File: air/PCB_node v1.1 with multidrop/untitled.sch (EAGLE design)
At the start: 113 parts, among them J1 10118193-0001LF, J2 10118193-0001LF, K1 351, K2 351, K3 SRD-05VDC-SL-C, K4 351, Q1 MMBT3904, Q10 S9013, Q2 MMBT3904, Q3 12MHz, Q4 S9013, Q5 S9013, Q6 S9013, Q7 12MHz, Q8 MMBT3904, Q9 MMBT3904, U1 CH340G, U10 ADS1115IDGSR, U11 PC817X2NIP0F, U2 ESP32-WROOM-32D, U3 AMS1117, U4 PC817X2NIP0F, U5 PC817X2NIP0F, U6 PC817X2NIP0F, U7 CH340G, U8 AMS1117, U9 ESP32-WROOM-32D, X1 MSTBA2, X2 MSTBA2, X3 MSTBA4, X4 MSTBA3, X5 MSTBA2, X6 MSTBA4, X7 C-GRID-02-70543, X8 MSTBA2

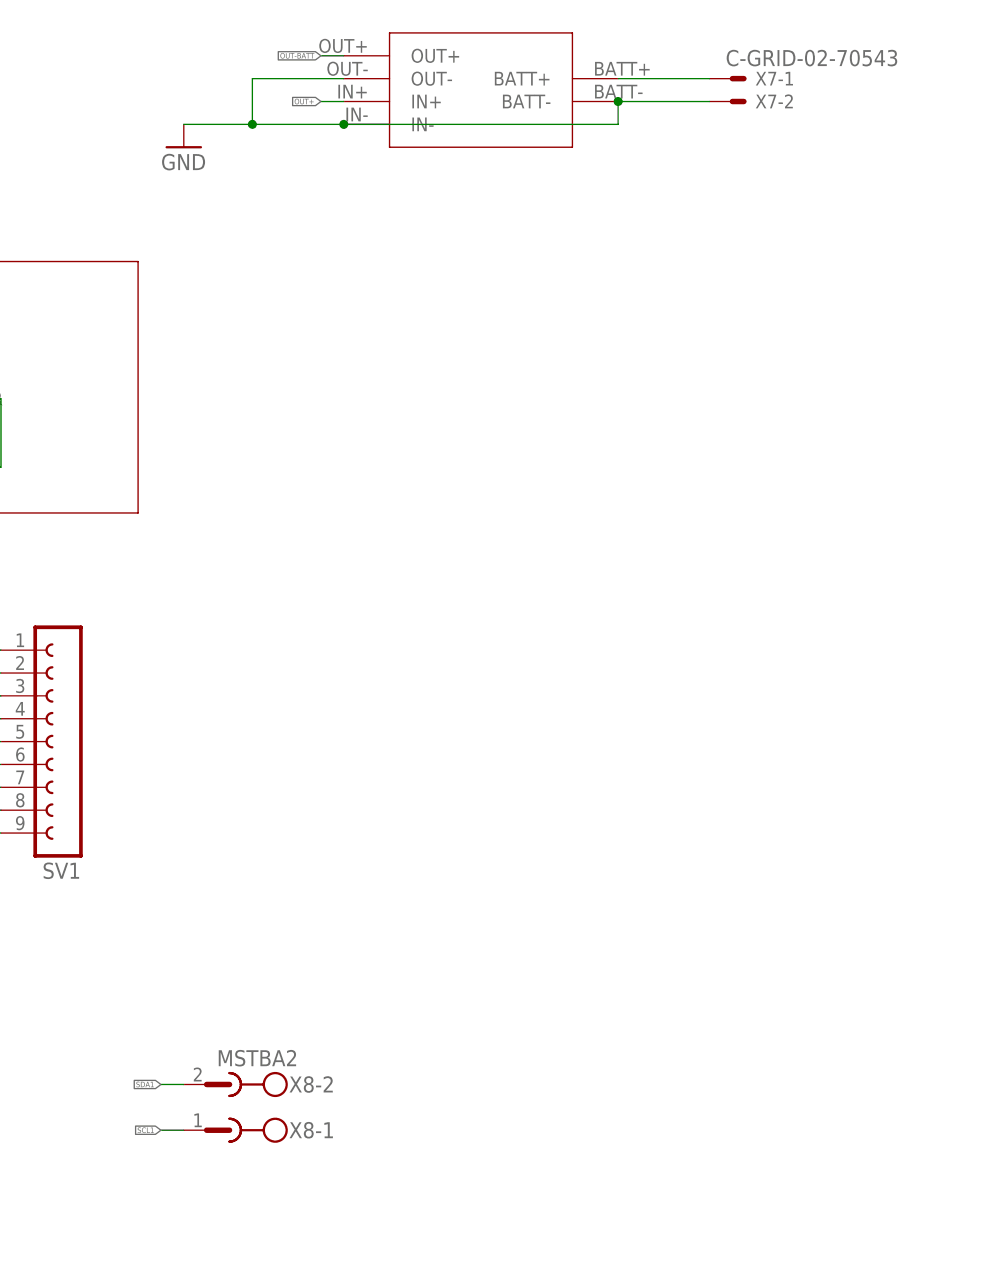
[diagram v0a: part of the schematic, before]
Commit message: menambah GPS chip
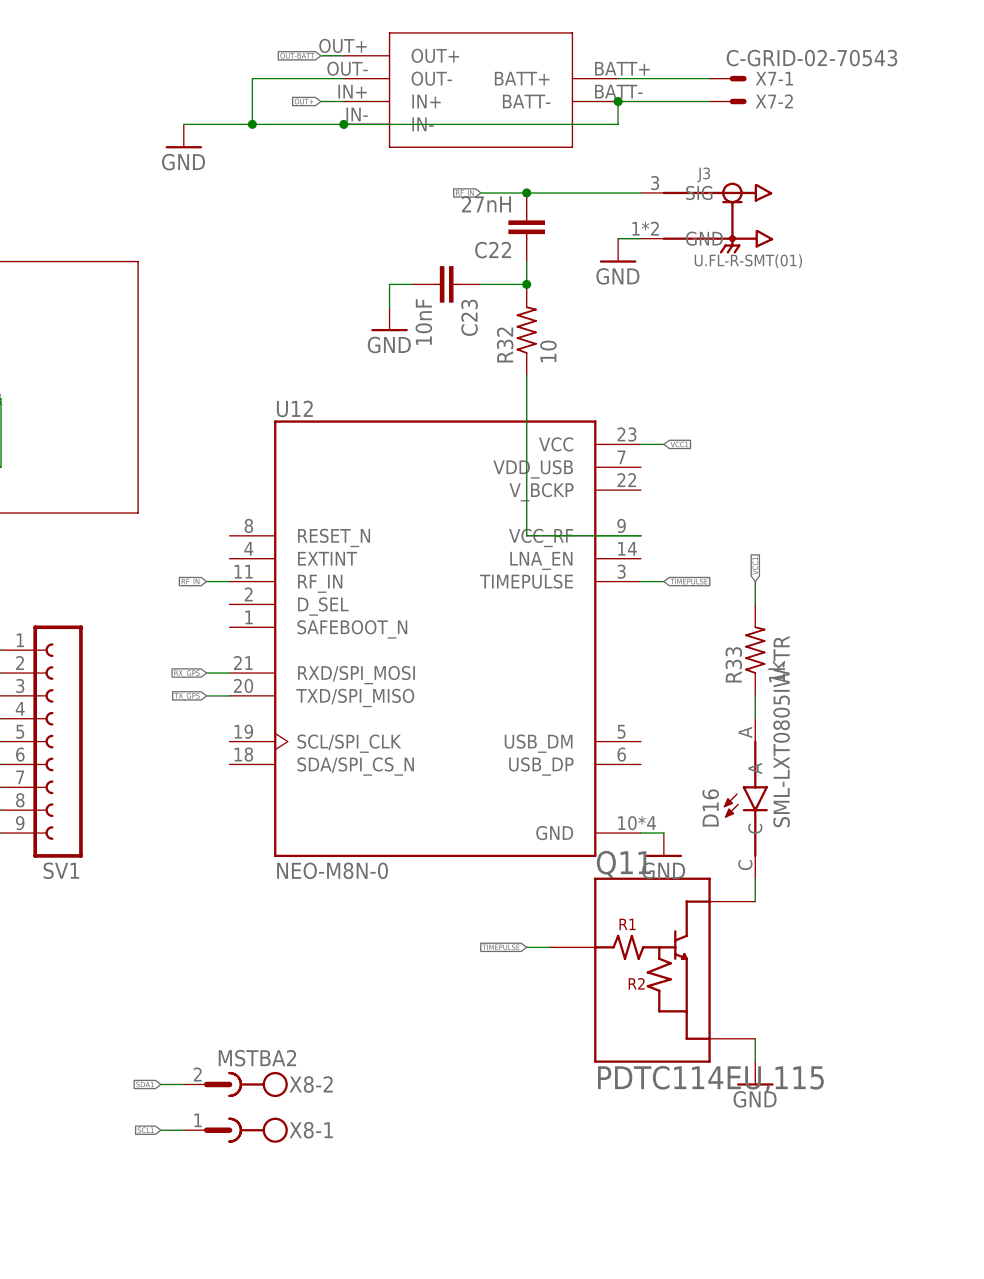
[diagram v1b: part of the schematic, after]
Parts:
- added C22: 27nH, rcl:C-EUC0805K
- added C23: 10nF, rcl:C-EUC0805K
- added D16: SML-LXT0805IW-TR, SML-LXT0805IW-TR:SML-LXT0805IW-TR
- added J3: U.FL-R-SMT(01), U.FL-R-SMT_01_:U.FL-R-SMT(01)
- added Q11: PDTC114EU,115, PDTC114EU_115:PDTC114EU,115
- added R32: 10, rcl:R-US_M0805
- added R33: 1k, rcl:R-US_M0805
- added U12: NEO-M8N-0, NEO-M8N-0:NEO-M8N-0
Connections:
- new net N$36: C22.1, C23.1, R32.2
- new net N$37: R32.1, U12.VCC_RF
- new net N$38: D16.C, Q11.OUTPUT
- new net N$39: D16.A, R33.1
- new net RF_IN: C22.2, J3.SIG, U12.RF_IN
- new net TIMEPULSE: Q11.INPUT, U12.TIMEPULSE
- net GND: now also C23.2, J3.GND, Q11.GND, U12.GND
- net RX_GPS: now also U12.RXD/SPI_MOSI
- net TX_GPS: now also U12.TXD/SPI_MISO
- net VCC1: now also R33.2, U12.VCC
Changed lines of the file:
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@@
 <part name="P+7" library="supply1" library_urn="urn:adsk.eagle:library:371" deviceset="VCC" device=""/>
 <part name="GND33" library="supply1" library_urn="urn:adsk.eagle:library:371" deviceset="GND" device=""/>
+<part name="U12" library="NEO-M8N-0" deviceset="NEO-M8N-0" device=""/>
+<part name="GND34" library="supply1" library_urn="urn:adsk.eagle:library:371" deviceset="GND" device=""/>
+<part name="J3" library="U.FL-R-SMT_01_" deviceset="U.FL-R-SMT(01)" device=""/>
+<part name="GND35" library="supply1" library_urn="urn:adsk.eagle:library:371" deviceset="GND" device=""/>
+<part name="C22" library="rcl" library_urn="urn:adsk.eagle:library:334" deviceset="C-EU" device="C0805K" package3d_urn="urn:adsk.eagle:package:23681/2" value="27nH"/>
+<part name="R32" library="rcl" library_urn="urn:adsk.eagle:library:334" deviceset="R-US_" device="M0805" package3d_urn="urn:adsk.eagle:package:23556/2" value="10"/>
+<part name="Q11" library="PDTC114EU_115" deviceset="PDTC114EU,115" device=""/>
+<part name="C23" library="rcl" library_urn="urn:adsk.eagle:library:334" deviceset="C-EU" device="C0805K" package3d_urn="urn:adsk.eagle:package:23681/2" value="10nF"/>
+<part name="GND36" library="supply1" library_urn="urn:adsk.eagle:library:371" deviceset="GND" device=""/>
+<part name="GND37" library="supply1" library_urn="urn:adsk.eagle:library:371" deviceset="GND" device=""/>
+<part name="D16" library="SML-LXT0805IW-TR" deviceset="SML-LXT0805IW-TR" device=""/>
+<part name="R33" library="rcl" library_urn="urn:adsk.eagle:library:334" deviceset="R-US_" device="M0805" package3d_urn="urn:adsk.eagle:package:23556/2" value="1k"/>
 </parts>
 <sheets>
@@
 <instance part="GND33" gate="1" x="78.74" y="172.72" smashed="yes">
 <attribute name="VALUE" x="76.2" y="170.18" size="1.778" layer="96"/>
+</instance>
+<instance part="U12" gate="G$1" x="287.02" y="99.06" smashed="yes">
+<attribute name="NAME" x="269.2361" y="122.4338" size="1.77845" layer="95"/>
+<attribute name="VALUE" x="269.2355" y="71.1126" size="1.77851875" layer="96"/>
+</instance>
+<instance part="GND34" gate="1" x="312.42" y="73.66" smashed="yes">
+<attribute name="VALUE" x="309.88" y="71.12" size="1.778" layer="96"/>
+</instance>
+<instance part="J3" gate="G$1" x="320.04" y="144.78" smashed="yes">
+<attribute name="NAME" x="316.22143125" y="148.85313125" size="1.27285" layer="95"/>
+<attribute name="VALUE" x="315.71218125" y="139.1793" size="1.27288125" layer="96"/>
+</instance>
+<instance part="GND35" gate="1" x="307.34" y="139.7" smashed="yes">
+<attribute name="VALUE" x="304.8" y="137.16" size="1.778" layer="96"/>
+</instance>
+<instance part="C22" gate="G$1" x="297.18" y="142.24" smashed="yes" rot="R180">
+<attribute name="NAME" x="295.656" y="141.859" size="1.778" layer="95" rot="R180"/>
+<attribute name="VALUE" x="295.656" y="146.939" size="1.778" layer="96" rot="R180"/>
+</instance>
+<instance part="R32" gate="G$1" x="297.18" y="132.08" smashed="yes" rot="R90">
+<attribute name="NAME" x="295.6814" y="128.27" size="1.778" layer="95" rot="R90"/>
+<attribute name="VALUE" x="300.482" y="128.27" size="1.778" layer="96" rot="R90"/>
+</instance>
+<instance part="Q11" gate="G$1" x="312.42" y="60.96" smashed="yes">
+<attribute name="NAME" x="304.7945" y="71.6357" size="2.54183125" layer="95"/>
+<attribute name="VALUE" x="304.79283125" y="47.7396" size="2.542390625" layer="96"/>
+</instance>
+<instance part="C23" gate="G$1" x="289.56" y="137.16" smashed="yes" rot="R270">
+<attribute name="NAME" x="289.941" y="135.636" size="1.778" layer="95" rot="R270"/>
+<attribute name="VALUE" x="284.861" y="135.636" size="1.778" layer="96" rot="R270"/>
+</instance>
+<instance part="GND36" gate="1" x="281.94" y="132.08" smashed="yes">
+<attribute name="VALUE" x="279.4" y="129.54" size="1.778" layer="96"/>
+</instance>
+<instance part="GND37" gate="1" x="322.58" y="48.26" smashed="yes">
+<attribute name="VALUE" x="320.04" y="45.72" size="1.778" layer="96"/>
+</instance>
+<instance part="D16" gate="G$1" x="322.58" y="78.74" smashed="yes" rot="R90">
+<attribute name="NAME" x="318.50973125" y="76.70486875" size="1.780740625" layer="95" rot="R90"/>
+<attribute name="VALUE" x="326.39315" y="76.70631875" size="1.77946875" layer="96" rot="R90"/>
+</instance>
+<instance part="R33" gate="G$1" x="322.58" y="96.52" smashed="yes" rot="R90">
+<attribute name="NAME" x="321.0814" y="92.71" size="1.778" layer="95" rot="R90"/>
+<attribute name="VALUE" x="325.882" y="92.71" size="1.778" layer="96" rot="R90"/>
 </instance>
 </instances>
@@
 <wire x1="91.44" y1="175.26" x2="78.74" y2="175.26" width="0.1524" layer="91"/>
 </segment>
+<segment>
+<pinref part="U12" gate="G$1" pin="GND"/>
+<wire x1="309.88" y1="76.2" x2="312.42" y2="76.2" width="0.1524" layer="91"/>
+<pinref part="GND34" gate="1" pin="GND"/>
+</segment>
+<segment>
+<pinref part="J3" gate="G$1" pin="GND"/>
+<wire x1="309.88" y1="142.24" x2="307.34" y2="142.24" width="0.1524" layer="91"/>
+<pinref part="GND35" gate="1" pin="GND"/>
+</segment>
+<segment>
+<pinref part="C23" gate="G$1" pin="2"/>
+<pinref part="GND36" gate="1" pin="GND"/>
+<wire x1="284.48" y1="137.16" x2="281.94" y2="137.16" width="0.1524" layer="91"/>
+<wire x1="281.94" y1="137.16" x2="281.94" y2="134.62" width="0.1524" layer="91"/>
+</segment>
+<segment>
+<pinref part="Q11" gate="G$1" pin="GND"/>
+<pinref part="GND37" gate="1" pin="GND"/>
+<wire x1="322.58" y1="53.34" x2="322.58" y2="50.8" width="0.1524" layer="91"/>
+</segment>
 </net>
 <net name="VUSB" class="0">
@@
 <label x="215.9" y="91.44" size="0.6096" layer="95" rot="R270" xref="yes"/>
 </segment>
+<segment>
+<pinref part="U12" gate="G$1" pin="VCC"/>
+<wire x1="309.88" y1="119.38" x2="312.42" y2="119.38" width="0.1524" layer="91"/>
+<label x="312.42" y="119.38" size="0.6096" layer="95" xref="yes"/>
+</segment>
+<segment>
+<pinref part="R33" gate="G$1" pin="2"/>
+<wire x1="322.58" y1="101.6" x2="322.58" y2="104.14" width="0.1524" layer="91"/>
+<label x="322.58" y="104.14" size="0.6096" layer="95" rot="R90" xref="yes"/>
+</segment>
 </net>
 <net name="RX_MICRO" class="0">
@@
 <label x="228.6" y="30.48" size="0.6096" layer="95" xref="yes"/>
 </segment>
+<segment>
+<pinref part="U12" gate="G$1" pin="RXD/SPI_MOSI"/>
+<wire x1="264.16" y1="93.98" x2="261.62" y2="93.98" width="0.1524" layer="91"/>
+<label x="261.62" y="93.98" size="0.6096" layer="95" rot="R180" xref="yes"/>
+</segment>
 </net>
 <net name="TX_GPS" class="0">
@@
 <wire x1="223.52" y1="45.72" x2="228.6" y2="45.72" width="0.1524" layer="91"/>
 <label x="228.6" y="45.72" size="0.6096" layer="95" xref="yes"/>
+</segment>
+<segment>
+<pinref part="U12" gate="G$1" pin="TXD/SPI_MISO"/>
+<wire x1="264.16" y1="91.44" x2="261.62" y2="91.44" width="0.1524" layer="91"/>
+<label x="261.62" y="91.44" size="0.6096" layer="95" rot="R180" xref="yes"/>
 </segment>
 </net>
@@
 </segment>
 </net>
+<net name="RF_IN" class="0">
+<segment>
+<pinref part="J3" gate="G$1" pin="SIG"/>
+<wire x1="309.88" y1="147.32" x2="297.18" y2="147.32" width="0.1524" layer="91"/>
+<pinref part="C22" gate="G$1" pin="2"/>
+<wire x1="297.18" y1="147.32" x2="292.1" y2="147.32" width="0.1524" layer="91"/>
+<junction x="297.18" y="147.32"/>
+<label x="292.1" y="147.32" size="0.6096" layer="95" rot="R180" xref="yes"/>
+</segment>
+<segment>
+<pinref part="U12" gate="G$1" pin="RF_IN"/>
+<wire x1="264.16" y1="104.14" x2="261.62" y2="104.14" width="0.1524" layer="91"/>
+<label x="261.62" y="104.14" size="0.6096" layer="95" rot="R180" xref="yes"/>
+</segment>
+</net>
+<net name="N$36" class="0">
+<segment>
+<pinref part="C22" gate="G$1" pin="1"/>
+<pinref part="R32" gate="G$1" pin="2"/>
+<wire x1="297.18" y1="139.7" x2="297.18" y2="137.16" width="0.1524" layer="91"/>
+<pinref part="C23" gate="G$1" pin="1"/>
+<wire x1="297.18" y1="137.16" x2="292.1" y2="137.16" width="0.1524" layer="91"/>
+<junction x="297.18" y="137.16"/>
+</segment>
+</net>
+<net name="N$37" class="0">
+<segment>
+<pinref part="R32" gate="G$1" pin="1"/>
+<pinref part="U12" gate="G$1" pin="VCC_RF"/>
+<wire x1="297.18" y1="127" x2="297.18" y2="109.22" width="0.1524" layer="91"/>
+<wire x1="297.18" y1="109.22" x2="309.88" y2="109.22" width="0.1524" layer="91"/>
+</segment>
+</net>
+<net name="TIMEPULSE" class="0">
+<segment>
+<pinref part="U12" gate="G$1" pin="TIMEPULSE"/>
+<wire x1="309.88" y1="104.14" x2="312.42" y2="104.14" width="0.1524" layer="91"/>
+<label x="312.42" y="104.14" size="0.6096" layer="95" xref="yes"/>
+</segment>
+<segment>
+<pinref part="Q11" gate="G$1" pin="INPUT"/>
+<wire x1="299.72" y1="63.5" x2="297.18" y2="63.5" width="0.1524" layer="91"/>
+<label x="297.18" y="63.5" size="0.6096" layer="95" rot="R180" xref="yes"/>
+</segment>
+</net>
+<net name="N$38" class="0">
+<segment>
+<pinref part="Q11" gate="G$1" pin="OUTPUT"/>
+<pinref part="D16" gate="G$1" pin="C"/>
+<wire x1="322.58" y1="68.58" x2="322.58" y2="71.12" width="0.1524" layer="91"/>
+</segment>
+</net>
+<net name="N$39" class="0">
+<segment>
+<pinref part="D16" gate="G$1" pin="A"/>
+<pinref part="R33" gate="G$1" pin="1"/>
+<wire x1="322.58" y1="88.9" x2="322.58" y2="91.44" width="0.1524" layer="91"/>
+</segment>
+</net>
